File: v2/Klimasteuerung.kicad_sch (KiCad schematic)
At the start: 35 parts, among them J1 Conn_01x07_Pin, Q1 2N3904, Q2 2N3906, Q3 2N3906, Q4 2N3904, Q5 2N3904, SW1 Override RPi, SW2 Override Windows, U1 74LS11, U2 74LS11

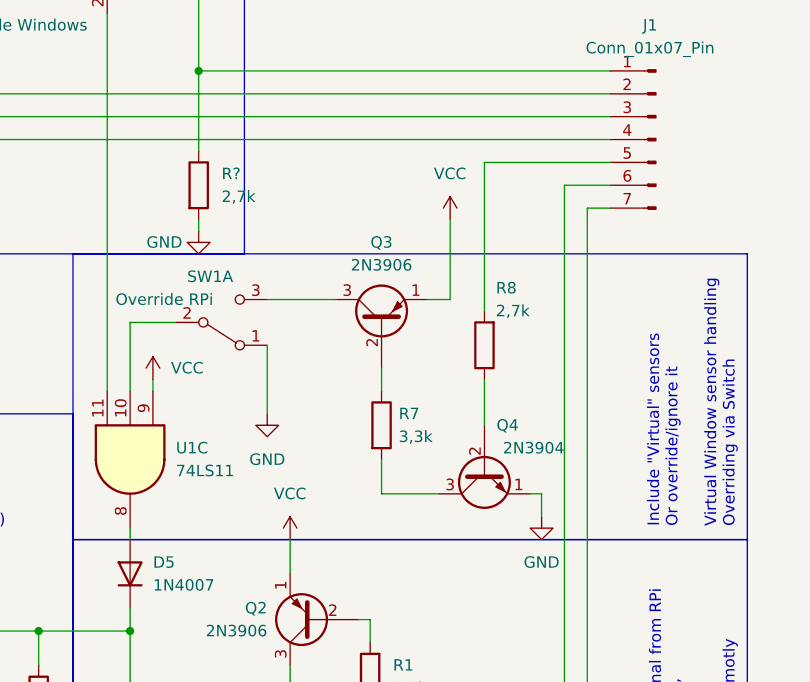
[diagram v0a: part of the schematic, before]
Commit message: updated
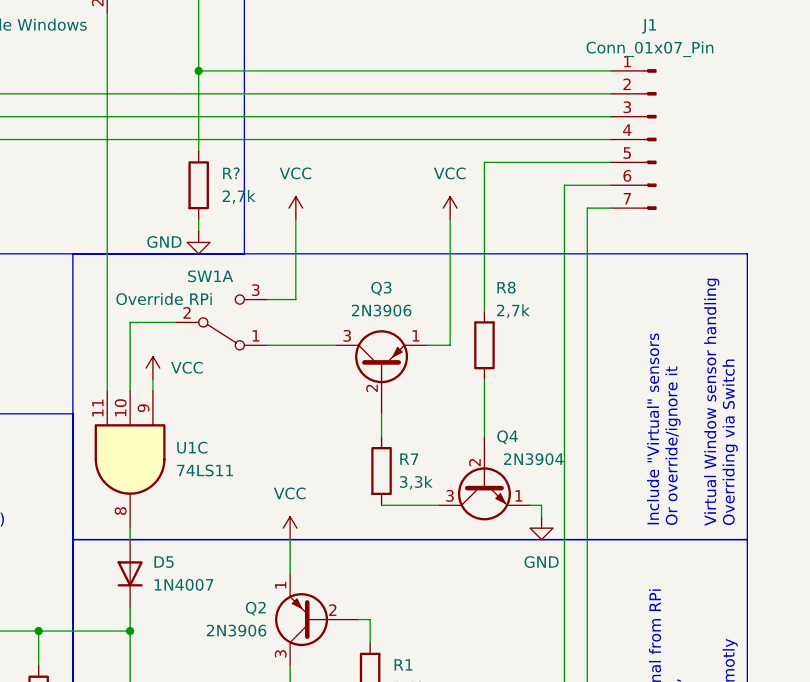
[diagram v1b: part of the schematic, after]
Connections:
- net GND: no longer SW1.1 (A)
- net VCC: now also SW1.3 (C)
- net at Q3.3 (C): now also SW1.1 (A); no longer SW1.3 (C)
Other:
- moved on the sheet: Q3, Q4, R7
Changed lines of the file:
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@@
+    (stroke (width 0) (type default))
+  )
+  (wire (pts (xy 134.62 102.87) (xy 137.795 102.87))
     (stroke (width 0) (type default))
   )
@@
     (stroke (width 0) (type default))
   )
-  (wire (pts (xy 134.62 107.95) (xy 134.62 115.57))
-    (stroke (width 0) (type default))
-  )
-  (wire (pts (xy 152.4 102.87) (xy 154.94 102.87))
+  (wire (pts (xy 152.4 107.95) (xy 154.94 107.95))
     (stroke (width 0) (type default))
   )
@@
     (stroke (width 0) (type default))
   )
-  (wire (pts (xy 147.32 110.49) (xy 147.32 113.03))
+  (wire (pts (xy 147.32 115.57) (xy 147.32 118.11))
     (stroke (width 0) (type default))
   )
@@
     (stroke (width 0) (type default))
   )
+  (wire (pts (xy 147.32 125.73) (xy 153.67 125.73))
+    (stroke (width 0) (type default))
+  )
   (wire (pts (xy 93.98 95.25) (xy 93.98 96.52))
     (stroke (width 0) (type default))
   )
-  (wire (pts (xy 154.94 102.87) (xy 154.94 93.98))
+  (wire (pts (xy 154.94 93.98) (xy 154.94 107.95))
     (stroke (width 0) (type default))
   )
@@
     (stroke (width 0) (type default))
   )
+  (wire (pts (xy 163.83 125.73) (xy 165.1 125.73))
+    (stroke (width 0) (type default))
+  )
   (wire (pts (xy 119.38 43.18) (xy 119.38 60.96))
     (stroke (width 0) (type default))
@@
     (stroke (width 0) (type default))
   )
-  (wire (pts (xy 163.83 124.46) (xy 165.1 124.46))
-    (stroke (width 0) (type default))
-  )
   (wire (pts (xy 158.75 104.14) (xy 158.75 87.63))
     (stroke (width 0) (type default))
   )
-  (wire (pts (xy 158.75 111.76) (xy 158.75 116.84))
-    (stroke (width 0) (type default))
-  )
-  (wire (pts (xy 134.62 102.87) (xy 142.24 102.87))
-    (stroke (width 0) (type default))
-  )
   (wire (pts (xy 81.28 80.01) (xy 81.28 87.63))
     (stroke (width 0) (type default))
   )
+  (wire (pts (xy 165.1 125.73) (xy 165.1 127))
+    (stroke (width 0) (type default))
+  )
   (wire (pts (xy 137.16 129.54) (xy 137.16 133.35))
     (stroke (width 0) (type default))
@@
     (stroke (width 0) (type default))
   )
-  (wire (pts (xy 153.67 124.46) (xy 147.32 124.46))
-    (stroke (width 0) (type default))
-  )
   (wire (pts (xy 49.53 139.7) (xy 53.34 139.7))
     (stroke (width 0) (type default))
@@
     (stroke (width 0) (type default))
   )
+  (wire (pts (xy 137.795 102.87) (xy 137.795 93.98))
+    (stroke (width 0) (type default))
+  )
   (wire (pts (xy 30.48 168.91) (xy 22.86 168.91))
     (stroke (width 0) (type default))
@@
     (stroke (width 0) (type default))
   )
-  (wire (pts (xy 165.1 124.46) (xy 165.1 127))
+  (wire (pts (xy 134.62 107.95) (xy 142.24 107.95))
     (stroke (width 0) (type default))
   )
@@
     (stroke (width 0) (type default))
   )
-  (wire (pts (xy 147.32 124.46) (xy 147.32 120.65))
+  (wire (pts (xy 158.75 111.76) (xy 158.75 118.11))
     (stroke (width 0) (type default))
   )
@@
     )
   )
-  (symbol (lib_id "Transistor_BJT:2N3904") (at 158.75 121.92 90) (mirror x) (unit 1)
-    (in_bom yes) (on_board yes) (dnp no)
-    (property "Reference" "Q4" (at 162.56 116.84 90)
-      (effects (font (size 1.27 1.27)) (justify left))
-    )
-    (property "Value" "2N3904" (at 167.64 119.38 90)
-      (effects (font (size 1.27 1.27)) (justify left))
-    )
-    (property "Footprint" "Package_TO_SOT_THT:TO-92_Inline" (at 160.655 127 0)
+  (symbol (lib_id "Transistor_BJT:2N3904") (at 158.75 123.19 90) (mirror x) (unit 1)
+    (in_bom yes) (on_board yes) (dnp no)
+    (property "Reference" "Q4" (at 162.56 118.11 90)
+      (effects (font (size 1.27 1.27)) (justify left))
+    )
+    (property "Value" "2N3904" (at 167.64 120.65 90)
+      (effects (font (size 1.27 1.27)) (justify left))
+    )
+    (property "Footprint" "Package_TO_SOT_THT:TO-92_Inline" (at 160.655 128.27 0)
       (effects (font (size 1.27 1.27) italic) (justify left) hide)
     )
-    (property "Datasheet" "https://www.onsemi.com/pub/Collateral/2N3903-D.PDF" (at 158.75 121.92 0)
+    (property "Datasheet" "https://www.onsemi.com/pub/Collateral/2N3903-D.PDF" (at 158.75 123.19 0)
       (effects (font (size 1.27 1.27)) (justify left) hide)
     )
@@
     )
   )
-  (symbol (lib_id "Device:R") (at 147.32 116.84 0) (unit 1)
-    (in_bom yes) (on_board yes) (dnp no) (fields_autoplaced)
-    (property "Reference" "R7" (at 149.225 115.57 0)
-      (effects (font (size 1.27 1.27)) (justify left))
-    )
-    (property "Value" "3,3k" (at 149.225 118.11 0)
-      (effects (font (size 1.27 1.27)) (justify left))
-    )
-    (property "Footprint" "" (at 145.542 116.84 90)
-      (effects (font (size 1.27 1.27)) hide)
-    )
-    (property "Datasheet" "~" (at 147.32 116.84 0)
+  (symbol (lib_id "Device:R") (at 147.32 121.92 0) (unit 1)
+    (in_bom yes) (on_board yes) (dnp no)
+    (property "Reference" "R7" (at 149.225 120.65 0)
+      (effects (font (size 1.27 1.27)) (justify left))
+    )
+    (property "Value" "3,3k" (at 149.225 123.19 0)
+      (effects (font (size 1.27 1.27)) (justify left))
+    )
+    (property "Footprint" "" (at 145.542 121.92 90)
+      (effects (font (size 1.27 1.27)) hide)
+    )
+    (property "Datasheet" "~" (at 147.32 121.92 0)
       (effects (font (size 1.27 1.27)) hide)
     )
@@
     )
   )
-  (symbol (lib_id "Transistor_BJT:2N3906") (at 147.32 105.41 90) (unit 1)
-    (in_bom yes) (on_board yes) (dnp no) (fields_autoplaced)
-    (property "Reference" "Q3" (at 147.32 96.52 90)
-      (effects (font (size 1.27 1.27)))
-    )
-    (property "Value" "2N3906" (at 147.32 99.06 90)
-      (effects (font (size 1.27 1.27)))
-    )
-    (property "Footprint" "Package_TO_SOT_THT:TO-92_Inline" (at 149.225 100.33 0)
+  (symbol (lib_id "Transistor_BJT:2N3906") (at 147.32 110.49 90) (unit 1)
+    (in_bom yes) (on_board yes) (dnp no) (fields_autoplaced)
+    (property "Reference" "Q3" (at 147.32 101.6 90)
+      (effects (font (size 1.27 1.27)))
+    )
+    (property "Value" "2N3906" (at 147.32 104.14 90)
+      (effects (font (size 1.27 1.27)))
+    )
+    (property "Footprint" "Package_TO_SOT_THT:TO-92_Inline" (at 149.225 105.41 0)
       (effects (font (size 1.27 1.27) italic) (justify left) hide)
     )
-    (property "Datasheet" "https://www.onsemi.com/pub/Collateral/2N3906-D.PDF" (at 147.32 105.41 0)
+    (property "Datasheet" "https://www.onsemi.com/pub/Collateral/2N3906-D.PDF" (at 147.32 110.49 0)
       (effects (font (size 1.27 1.27)) (justify left) hide)
     )
@@
         (path "/e63e39d7-6ac0-4ffd-8aa3-1841a4541b55"
           (reference "Q3") (unit 1)
+        )
+      )
+    )
+  )
+  (symbol (lib_id "power:VCC") (at 137.795 93.98 0) (unit 1)
+    (in_bom yes) (on_board yes) (dnp no) (fields_autoplaced)
+    (property "Reference" "#PWR06" (at 137.795 97.79 0)
+      (effects (font (size 1.27 1.27)) hide)
+    )
+    (property "Value" "VCC" (at 137.795 88.9 0)
+      (effects (font (size 1.27 1.27)))
+    )
+    (property "Footprint" "" (at 137.795 93.98 0)
+      (effects (font (size 1.27 1.27)) hide)
+    )
+    (property "Datasheet" "" (at 137.795 93.98 0)
+      (effects (font (size 1.27 1.27)) hide)
+    )
+    (pin "1")
+    (instances
+      (project "Klimasteuerung"
+        (path "/e63e39d7-6ac0-4ffd-8aa3-1841a4541b55"
+          (reference "#PWR06") (unit 1)
         )
       )
@@
         )
       )
-    )
-  )
-  (symbol (lib_id "power:GND") (at 134.62 115.57 0) (unit 1)
-    (in_bom yes) (on_board yes) (dnp no) (fields_autoplaced)
-    (property "Reference" "#PWR06" (at 134.62 121.92 0)
-      (effects (font (size 1.27 1.27)) hide)
-    )
-    (property "Value" "GND" (at 134.62 120.65 0)
-      (effects (font (size 1.27 1.27)))
-    )
-    (property "Footprint" "" (at 134.62 115.57 0)
-      (effects (font (size 1.27 1.27)) hide)
-    )
-    (property "Datasheet" "" (at 134.62 115.57 0)
-      (effects (font (size 1.27 1.27)) hide)
-    )
-    (pin "1")
-    (instances
-      (project "Klimasteuerung"
-        (path "/e63e39d7-6ac0-4ffd-8aa3-1841a4541b55"
-          (reference "#PWR06") (unit 1)
-        )
-      )

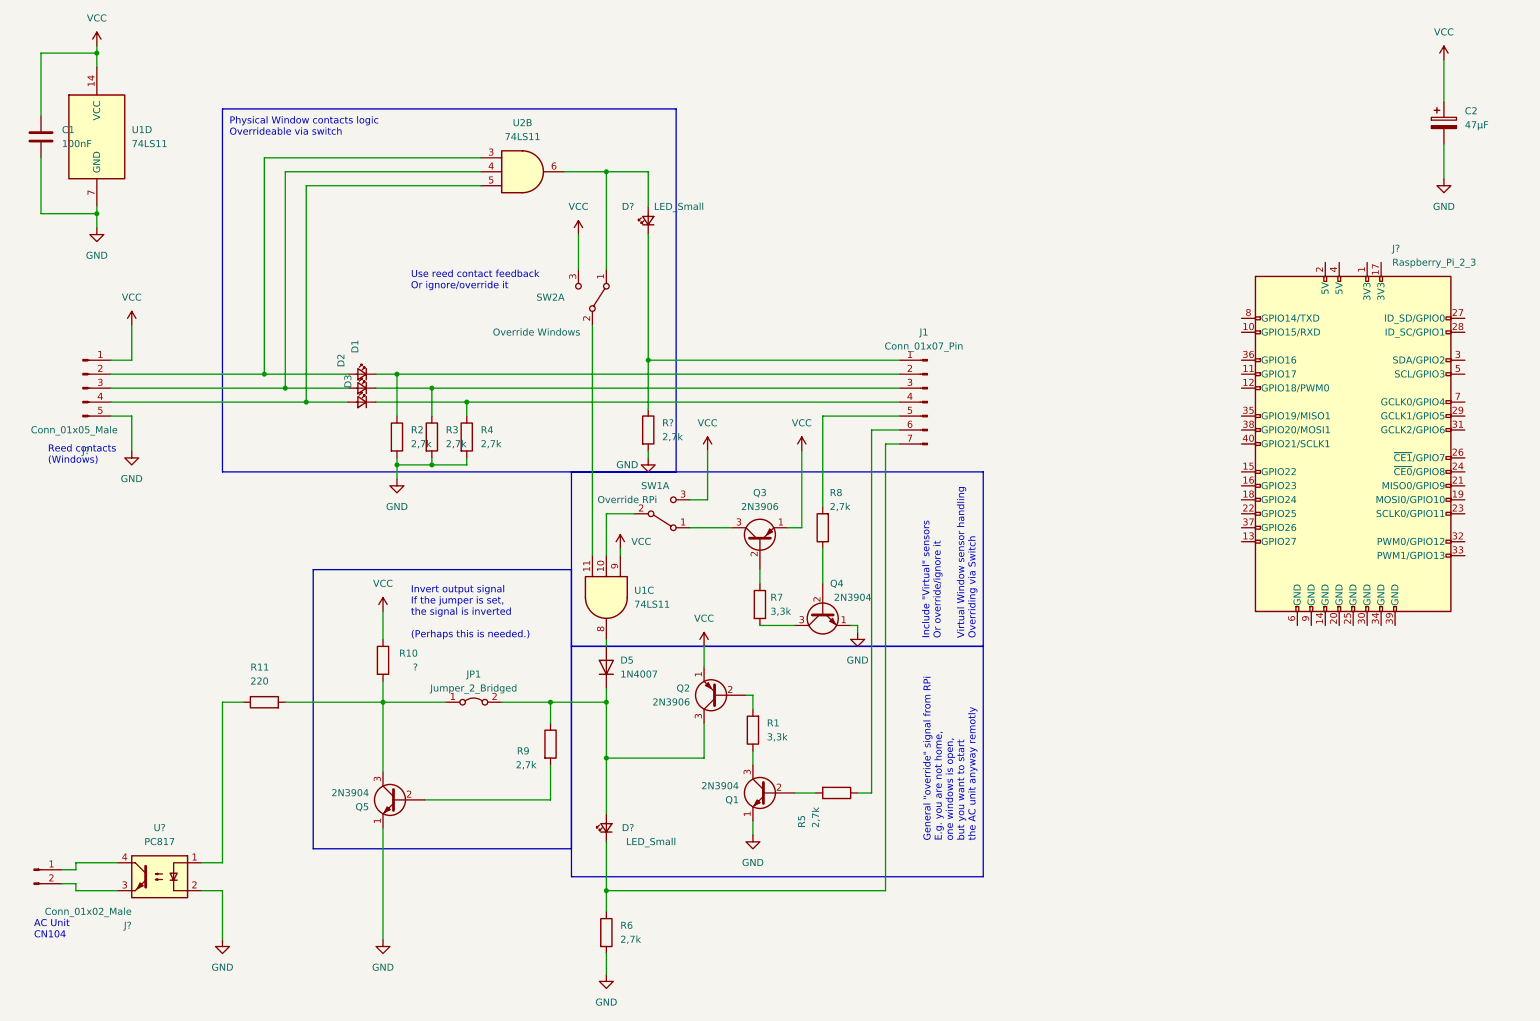
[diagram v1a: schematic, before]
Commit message: adjustments to schematic
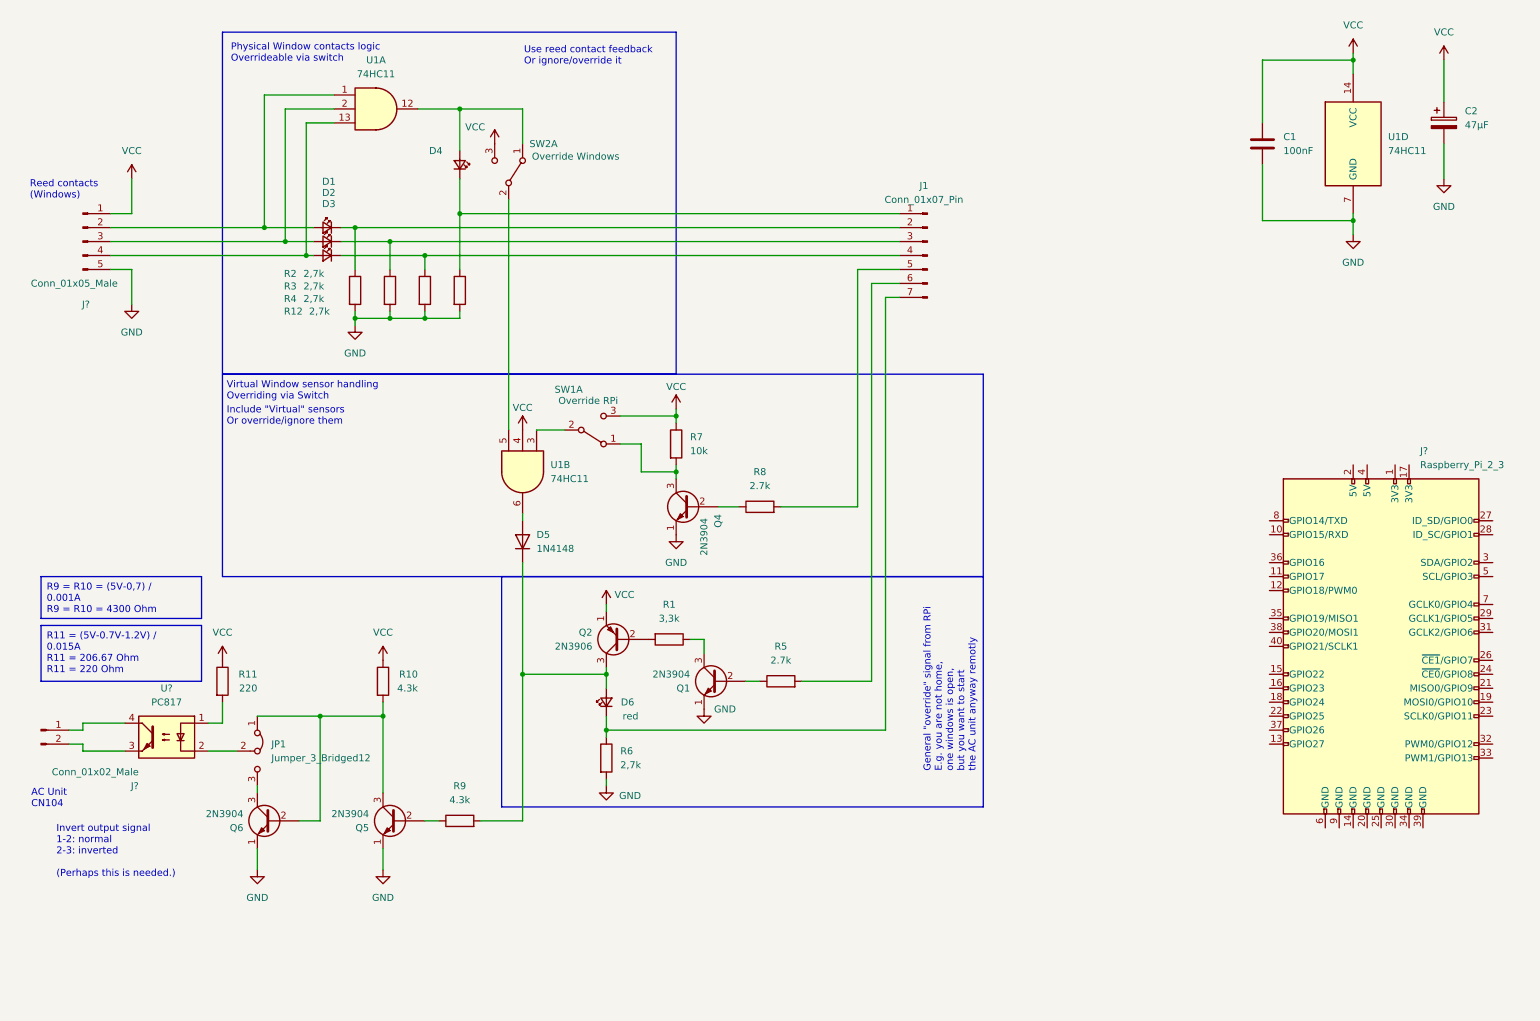
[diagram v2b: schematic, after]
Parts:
- removed D5: 1N4007, Diode_THT:D_DO-41_SOD81_P10.16mm_Horizontal, symbol Diode:1N4007
- removed D? (x2): LED_Small, symbol Device:LED_Small
- removed JP1: Jumper_2_Bridged, symbol Jumper:Jumper_2_Bridged
- removed Q3: 2N3906, Package_TO_SOT_THT:TO-92_Inline, symbol Transistor_BJT:2N3906
- removed R?: 2,7k, symbol Device:R
- removed unit 3 of U1
- removed U2: 74LS11, symbol 74xx:74LS11
- added D4, D6: red, symbol Device:LED_Small
- added D5: 1N4148, Diode_THT:D_DO-35_SOD27_P7.62mm_Horizontal, symbol Diode:1N4148
- added JP1: Jumper_3_Bridged12, symbol Jumper:Jumper_3_Bridged12
- added Q6: 2N3904, Package_TO_SOT_THT:TO-92_Inline, symbol Transistor_BJT:2N3904
- added R12: 2,7k, symbol Device:R
- added unit 2 of U1
- added unit 1 of U1
- D1, D2, D3: value LED_Small -> red
- R10: value ? -> 4.3k
- R5, R8: value 2,7k -> 2.7k
- R7: value 3,3k -> 10k
- R9: value 2,7k -> 4.3k
- U1: value 74LS11 -> 74HC11
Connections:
- net GND: now also Q6.1 (E), R12.2; no longer U?.2
- net VCC: now also R11.1, R7.1, U1.4
- net at U?.1: now also R11.2; no longer R11.1
- net at R5.1: now also Q1.2 (B); no longer J1.6 (Pin_6)
- net at R5.2: now also J1.6 (Pin_6); no longer Q1.2 (B)
- net at D2.2 (A), J?.3 (Pin_3): now also U1.2
- net at Q2.3 (C): now also R9.2, D5.1 (K), D6.2 (A); no longer R9.1
- net at J1.7 (Pin_7), R6.1: now also D6.1 (K)
- net at Q5.3 (C), R10.2: now also JP1.1 (A), Q6.2 (B); no longer R11.2
- net at J1.1 (Pin_1): now also D4.1 (K), R12.1
- net at SW2.1 (A): now also D4.2 (A), U1.12
- net at Q4.3 (C), R7.2: now also SW1.1 (A)
- net at SW2.2 (B): now also U1.5
- net at D1.2 (A), J?.2 (Pin_2): now also U1.1
- net at D3.2 (A), J?.4 (Pin_4): now also U1.13
- net at Q5.2 (B): now also R9.1; no longer R9.2
- net at SW1.2 (B): now also U1.3
- new net: JP1.2 (C), U?.2
- new net: JP1.3 (B), Q6.3 (C)
- new net: D5.2 (A), U1.6
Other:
- note added: "Include "Virtual" sensors Or override/ignore them"
- note added: "Invert output signal 1-2: normal 2-3: inverted (Perhaps this is needed.)"
- note removed: "Include "Virtual" sensors Or override/ignore it"
- note removed: "Invert output signal If the jumper is set, the signal is inverted (Perhaps this is needed.)"
- moved on the sheet: C1, D1, D2, D3, J1, J?, Q1, Q2, Q4, Q5, R1, R10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
